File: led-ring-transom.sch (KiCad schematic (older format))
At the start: 68 parts

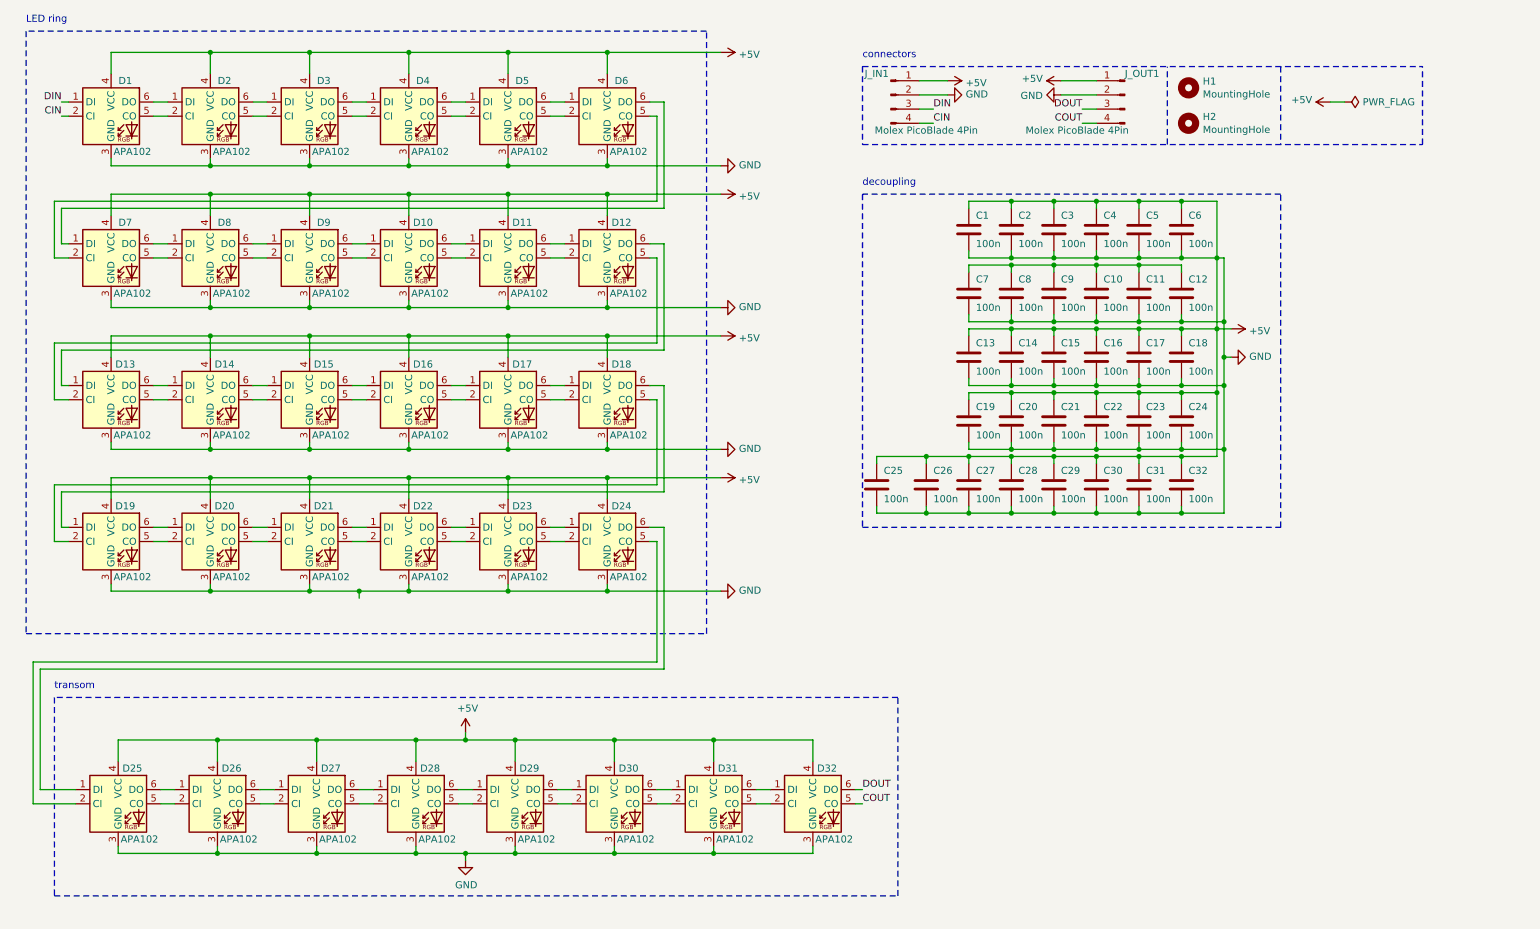
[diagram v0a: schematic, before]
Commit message: Finish PCB
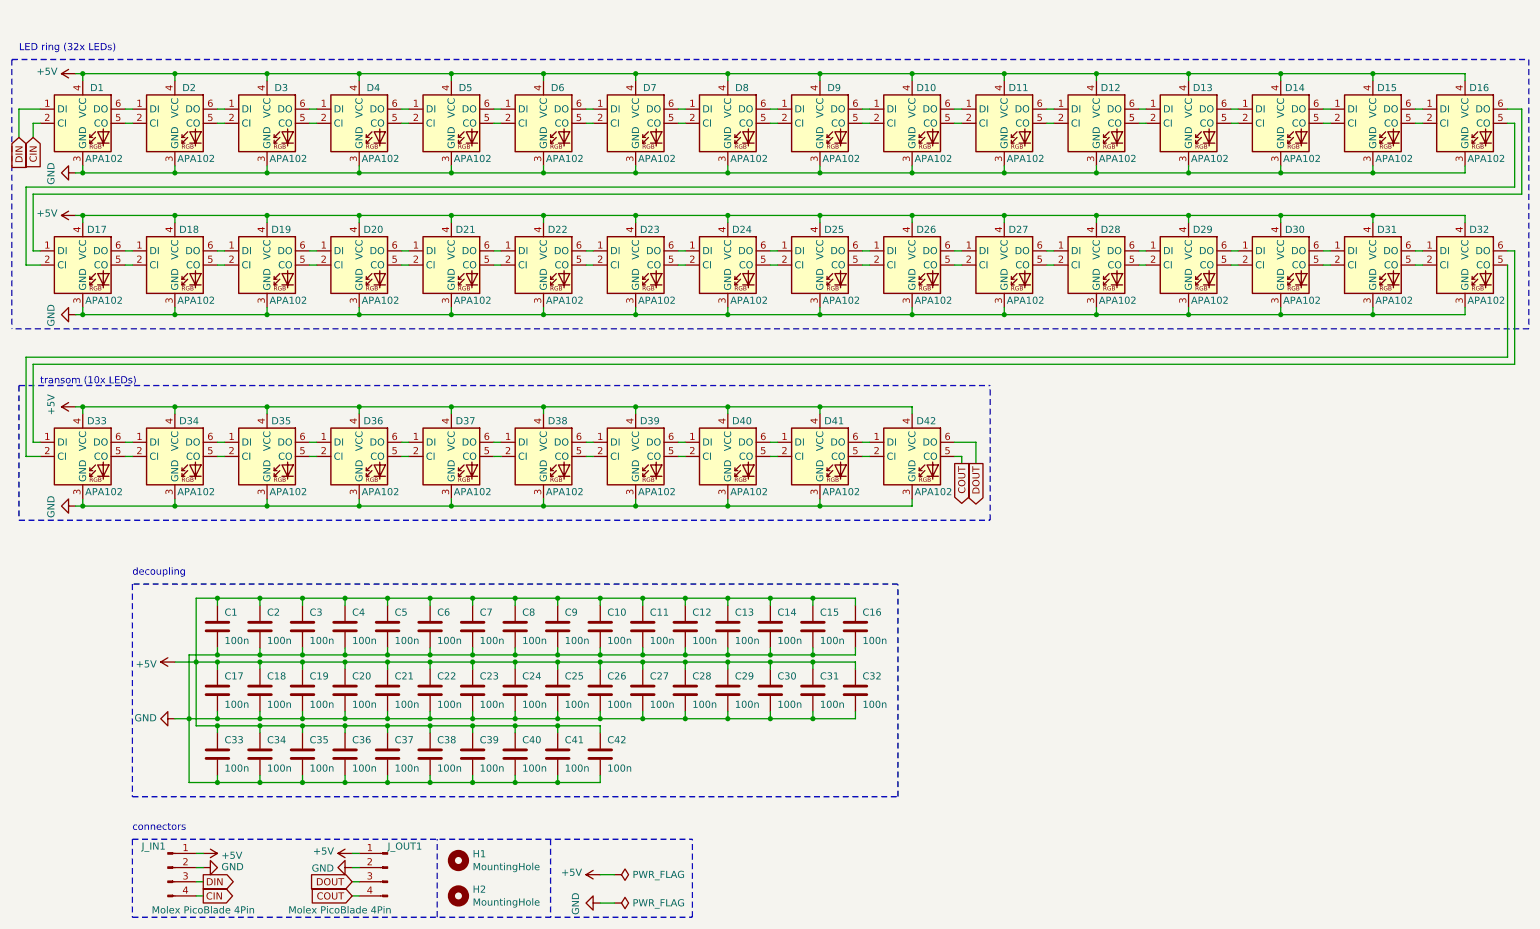
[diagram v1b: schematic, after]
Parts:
- added C33, C34, C35, C36, C37, C38, C39, C40, C41, C42: 100n, Capacitor_SMD:C_0603_1608Metric, symbol Device:C
- added D13, D14, D15, D16, D29, D30, D31, D32, D41, D42: APA102, LED_SMD:LED_RGB_5050-6, symbol LED:APA102
- H1, H2: footprint (none) -> extraFootprints:MountingHole_3.2mm_M3_ISO7380_Keepout
- J_IN1, J_OUT1: footprint Connector_Molex:Molex_PicoBlade_53261-0471_1x04-1MP_P1.25mm_Horizontal -> Connector_Molex:Molex_PicoBlade_53047-0410_1x04_P1.25mm_Vertical
- renumbered C29 to C25, C30 to C26, C31 to C27, C32 to C28, C25 to C29, C26 to C30, C27 to C31, C28 to C32, D13 to D17, D14 to D18, D15 to D19, D16 to D20, D17 to D21, D18 to D22, D19 to D23, D20 to D24, D21 to D25, D22 to D26, D23 to D27, D24 to D28, D25 to D33, D26 to D34, D27 to D35, D28 to D36, D29 to D37, D30 to D38, D31 to D39, D32 to D40
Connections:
- net +5V: now also C10.1, C11.1, C12.1, C7.1, C8.1, C9.1, C33.1, C34.1, C35.1, C36.1, C37.1, C38.1, C39.1, C40.1, C41.1, C42.1, D13.4 (VCC), D14.4 (VCC), D15.4 (VCC), D16.4 (VCC), D29.4 (VCC), D30.4 (VCC), D31.4 (VCC), D32.4 (VCC), D41.4 (VCC), D42.4 (VCC); no longer C1.2, C10.2, C11.2, C12.2, C13.2, C14.2, C15.2, C16.2, C17.2, C18.2, C19.2, C2.2, C20.2, C21.2, C22.2, C23.2, C24.2, C25.2, C26.2, C27.2, C28.2, C29.2, C3.2, C30.2, C31.2, C32.2, C4.2, C5.2, C6.2, C7.2, C8.2, C9.2, D1.3 (GND), D10.3 (GND), D11.3 (GND), D12.3 (GND), D17.3 (GND), D18.3 (GND), D19.3 (GND), D2.3 (GND), D20.3 (GND), D21.3 (GND), D22.3 (GND), D23.3 (GND), D24.3 (GND), D25.3 (GND), D26.3 (GND), D27.3 (GND), D28.3 (GND), D3.3 (GND), D33.3 (GND), D34.3 (GND), D35.3 (GND), D36.3 (GND), D37.3 (GND), D38.3 (GND), D39.3 (GND), D4.3 (GND), D40.3 (GND), D5.3 (GND), D6.3 (GND), D7.3 (GND), D8.3 (GND), D9.3 (GND), J_IN1.2 (Pin_2), J_OUT1.2 (Pin_2)
- net COUT: now also D42.5 (CO); no longer D40.5 (CO)
- net DOUT: now also D42.6 (DO); no longer D40.6 (DO)
- net at D33.1 (DI): now also D32.6 (DO); no longer D28.6 (DO)
- net at D33.2 (CI): now also D32.5 (CO); no longer D28.5 (CO)
- net at D17.1 (DI): now also D16.6 (DO); no longer D12.6 (DO)
- net at D17.2 (CI): now also D16.5 (CO); no longer D12.5 (CO)
- new net: D40.5 (CO), D41.2 (CI)
- new net: D40.6 (DO), D41.1 (DI)
- new net: D28.5 (CO), D29.2 (CI)
- new net: D28.6 (DO), D29.1 (DI)
- new net: D12.5 (CO), D13.2 (CI)
- new net: D12.6 (DO), D13.1 (DI)
- new net: D13.5 (CO), D14.2 (CI)
- new net: D13.6 (DO), D14.1 (DI)
- new net: D14.5 (CO), D15.2 (CI)
- new net: D14.6 (DO), D15.1 (DI)
- new net: D15.5 (CO), D16.2 (CI)
- new net: D15.6 (DO), D16.1 (DI)
- new net: D29.5 (CO), D30.2 (CI)
- new net: D29.6 (DO), D30.1 (DI)
- new net: D30.5 (CO), D31.2 (CI)
- new net: D30.6 (DO), D31.1 (DI)
- new net: D31.5 (CO), D32.2 (CI)
- new net: D31.6 (DO), D32.1 (DI)
- new net: D41.5 (CO), D42.2 (CI)
- new net: D41.6 (DO), D42.1 (DI)
- new net GND: C1.2, C10.2, C11.2, C12.2, C13.2, C14.2, C15.2, C16.2, C17.2, C18.2, C19.2, C2.2, C20.2, C21.2, C22.2, C23.2, C24.2, C25.2, C26.2, C27.2, C28.2, C29.2, C3.2, C30.2, C31.2, C32.2, C33.2, C34.2, C35.2, C36.2, C37.2, C38.2, C39.2, C4.2, C40.2, C41.2, C42.2, C5.2, C6.2, C7.2, C8.2, C9.2, D1.3 (GND), D10.3 (GND), D11.3 (GND), D12.3 (GND), D13.3 (GND), D14.3 (GND), D15.3 (GND), D16.3 (GND), D17.3 (GND), D18.3 (GND), D19.3 (GND), D2.3 (GND), D20.3 (GND), D21.3 (GND), D22.3 (GND), D23.3 (GND), D24.3 (GND), D25.3 (GND), D26.3 (GND), D27.3 (GND), D28.3 (GND), D29.3 (GND), D3.3 (GND), D30.3 (GND), D31.3 (GND), D32.3 (GND), D33.3 (GND), D34.3 (GND), D35.3 (GND), D36.3 (GND), D37.3 (GND), D38.3 (GND), D39.3 (GND), D4.3 (GND), D40.3 (GND), D41.3 (GND), D42.3 (GND), D5.3 (GND), D6.3 (GND), D7.3 (GND), D8.3 (GND), D9.3 (GND), J_IN1.2 (Pin_2), J_OUT1.2 (Pin_2)
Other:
- note added: "LED ring (32x LEDs)"
- note added: "transom (10x LEDs)"
- note removed: "LED ring"
- note removed: "transom"
- moved on the sheet: C1, C10, C11, C12, C13, C14, C15, C16, C17, C18, C19, C2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
